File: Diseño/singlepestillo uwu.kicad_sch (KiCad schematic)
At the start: 17 parts, among them J1 MAX98357A, J2 Conn_01x03_Pin, J3 Screw_Terminal_01x03, J5 Screw_Terminal_01x02, J9 Screw_Terminal_01x03, K3 G6AU, Q6 MMBT2222A, U3 EL817, U5 L7805, U6 ESP32DevKitv1

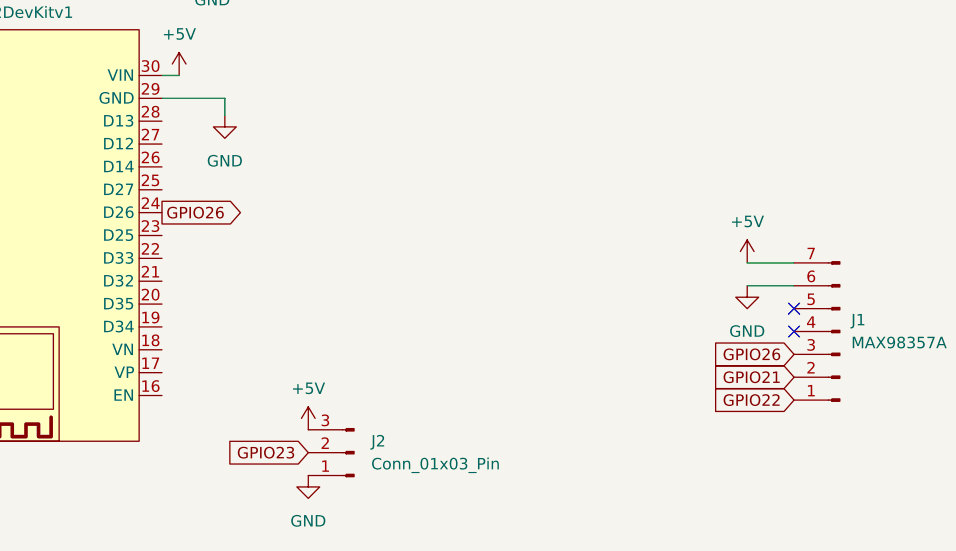
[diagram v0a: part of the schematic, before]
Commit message: Primer modelo final pcb
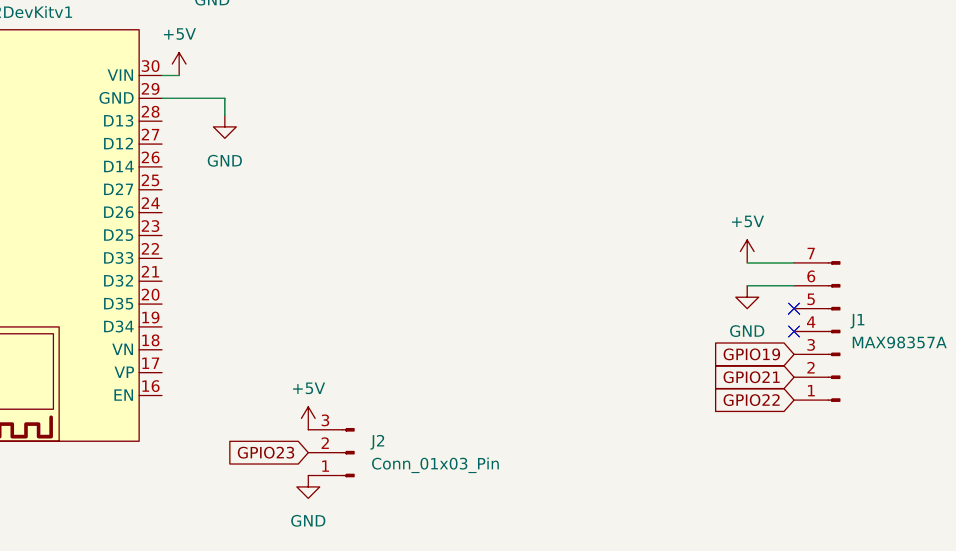
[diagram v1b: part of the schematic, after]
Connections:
- net GPIO19: now also J1.3 (Pin_3)
- net GPIO26: no longer names the net of U6.24 (D26)
- net GPIO26: no longer J1.3 (Pin_3)
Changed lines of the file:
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@@
-		)
-	)
-	(global_label "GPIO26"
-		(shape output)
-		(at 66.04 72.39 0)
-		(fields_autoplaced yes)
-		(effects
-			(font
-				(size 1.27 1.27)
-			)
-			(justify left)
-		)
-		(property "Intersheetrefs" "${INTERSHEET_REFS}"
-			(at 75.9195 72.39 0)
-			(effects
-				(font
-					(size 1.27 1.27)
-				)
-				(justify left)
-				(hide yes)
-			)
 		)
 	)
@@
 		)
 	)
-	(global_label "GPIO26"
+	(global_label "GPIO19"
 		(shape input)
 		(at 136.271 88.138 180)
